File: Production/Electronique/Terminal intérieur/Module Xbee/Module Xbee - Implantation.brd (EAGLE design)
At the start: 48 x 38.5 mm, 7 parts, among them U100 XBEE, U201 COMMUTATEUR_GLISSIERE_1RT_100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, U202 MCP1700T-3302E/TT

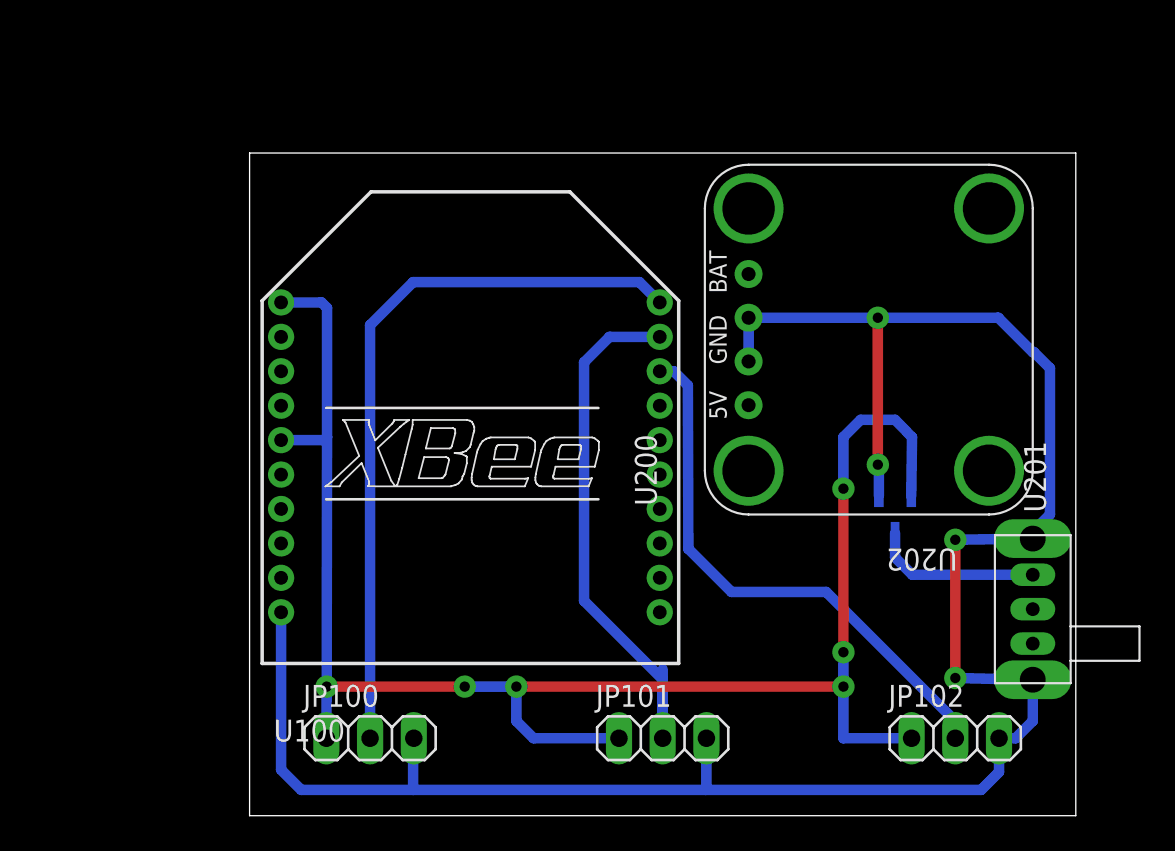
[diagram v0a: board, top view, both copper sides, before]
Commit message: Premiere reorganisation
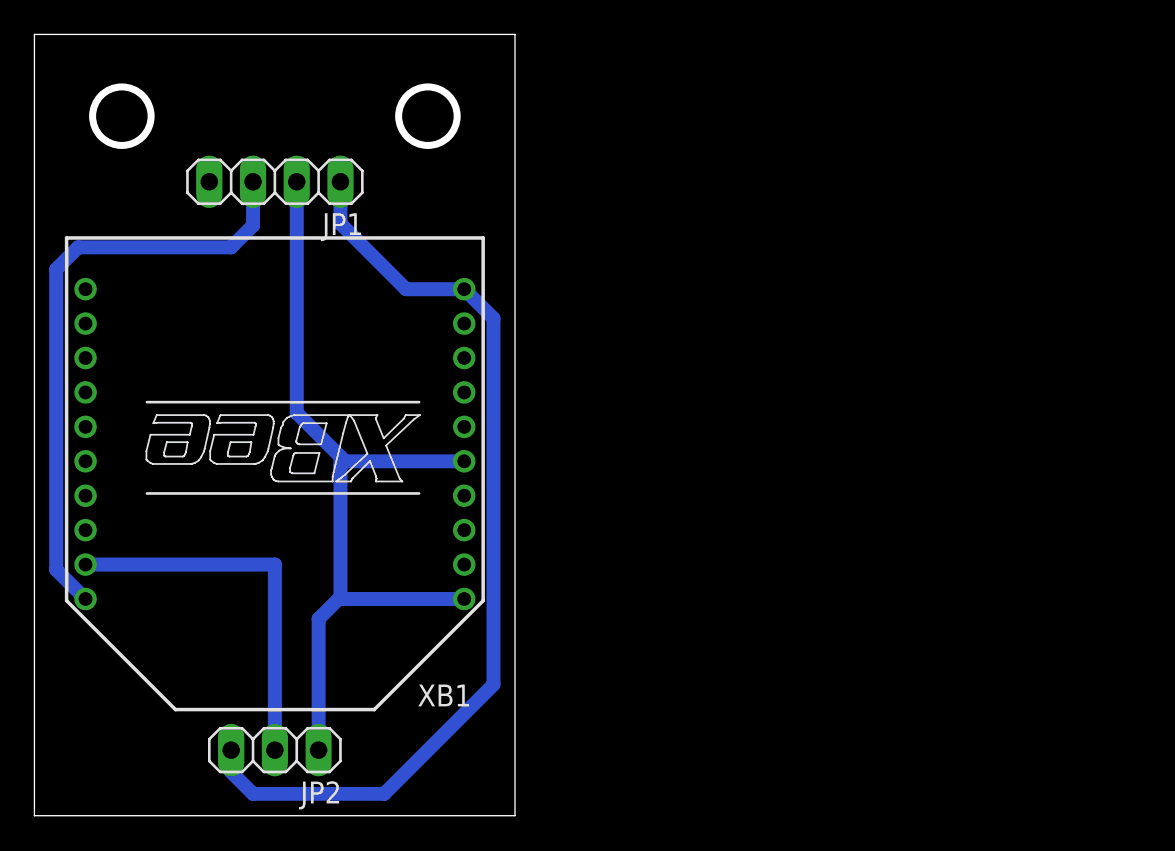
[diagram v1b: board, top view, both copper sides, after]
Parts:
- removed JP100: CAPT0, pinhead:1X03
- removed JP101: CAPT1, pinhead:1X03
- removed JP102: CAPT2, pinhead:1X03
- removed U100: XBEE, Eagle_UOF_Lib:XBEE
- removed U200: (no value), Eagle_UOF_Lib:MICROUSB-LIPO-CHARGEUR-ADAFRUIT
- removed U201: COMMUTATEUR_GLISSIERE_1RT_100MA, Eagle_UOF_Lib:COMMUTATEUR_GLISSIERE_1RT_100MA
- removed U202: MCP1700T-3302E/TT, Eagle_UOF_Lib:SOT95P237X112-3N
- added JP1: (no value), pinhead:1X04
- added JP2: (no value), pinhead:1X03
- added XB1: XBEE, maxstream:XBEE
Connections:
- removed net 3V3: JP100.1, JP101.1, JP102.1, U100.1, U100.5, U202.2
- removed net GND: JP100.3, JP101.3, JP102.3, U100.10, U200.GND1, U200.GND2, U201.GNDA, U201.GNDB, U202.1
- removed net N$7: JP101.2, U100.19
- removed net N$8: U201.OUTA, U202.3
- removed net N$9: JP102.2, U100.18
- new net N$3: JP1.3, XB1.20
- new net N$4: JP2.2, XB1.19
- net N$1: now also JP1.2, JP2.1, XB1.1, XB1.5; no longer JP100.2, U100.20
- net N$2: now also JP1.1, JP2.3, XB1.10; no longer U200.BAT, U201.COM
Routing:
- net GND: track 123.6 -> 0.00 mm, vias 4 -> 0
- net 3V3: track 98.6 -> 0.00 mm, vias 6 -> 0
- net N$2: track 0.00 -> 54.5 mm
- net N$3: track 0.00 -> 34.9 mm
- net N$7: track 32.7 -> 0.00 mm
- net N$9: track 32.1 -> 0.00 mm
- net N$4: track 0.00 -> 21.8 mm
- net N$8: track 9.82 -> 0.00 mm
- net N$1: track 42.4 -> 49.6 mm
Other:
- board size 48 x 38.5 mm -> 27.9 x 45.4 mm
